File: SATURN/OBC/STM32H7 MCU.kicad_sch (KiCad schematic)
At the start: 16 parts, among them IC1 STM32H735AGI6, IC2 STM32H735AGI6

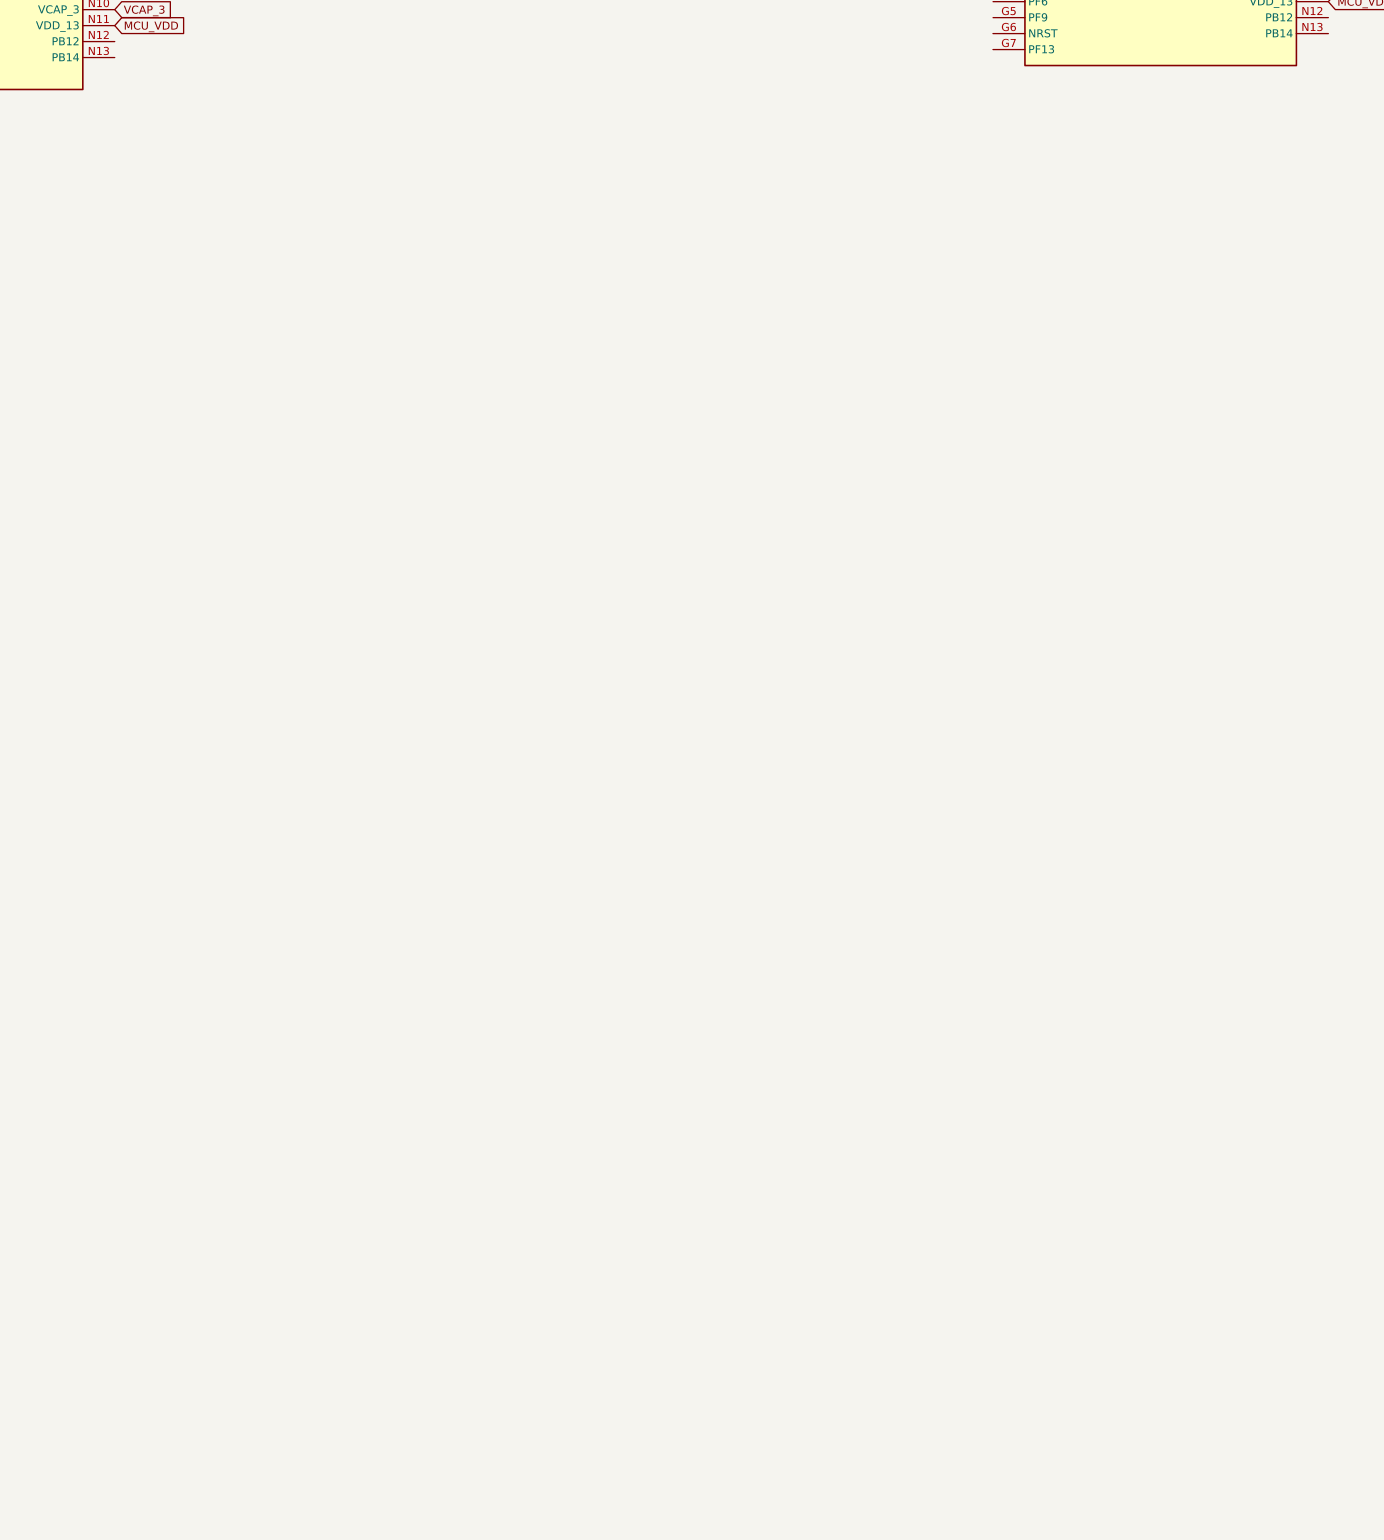
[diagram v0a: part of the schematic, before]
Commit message: a
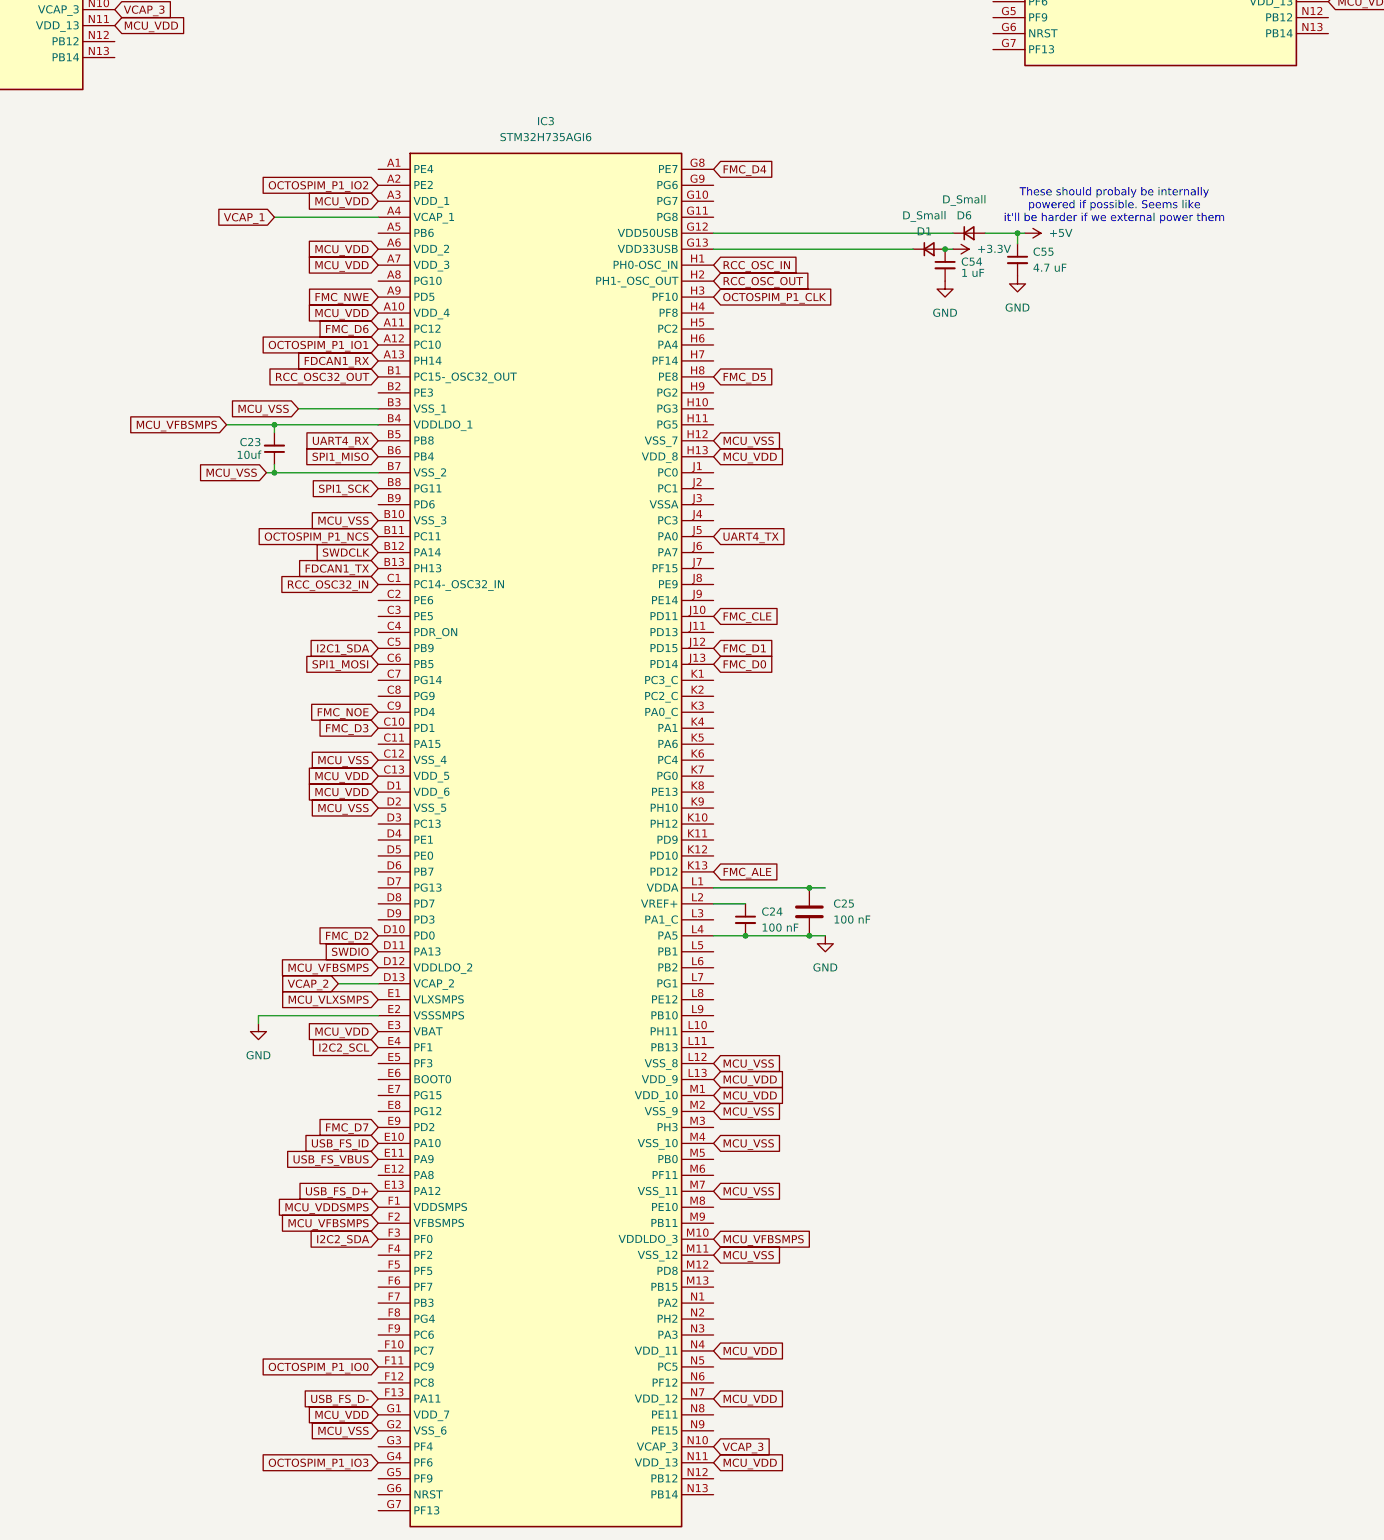
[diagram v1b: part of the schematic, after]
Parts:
- added C23: 10uf, Capacitor_SMD:C_0603_1608Metric, symbol Device:C_Small
- added C24: 100 nF, symbol Device:C_Small
- added C25: 100 nF, symbol Device:C
- added C54: 1 uF, symbol Device:C_Small
- added C55: 4.7 uF, symbol Device:C_Small
- added D1, D6: D_Small, symbol Device:D_Small
- added IC3: STM32H735AGI6, Gabriel_footprints:BGA169C50P13X13_700X700X60, symbol STM32H735AGI6:STM32H735AGI6
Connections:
- net +3.3V: now also C54.1, D1.2 (A)
- net +5V: now also C55.1, D6.2 (A)
- net GND: now also C24.2, C25.2, C54.2, C55.2, IC3.E2 (VSSSMPS), IC3.L4 (PA5)
- net MCU_VDD: now also IC3.A10 (VDD_4), IC3.A3 (VDD_1), IC3.A6 (VDD_2), IC3.A7 (VDD_3), IC3.C13 (VDD_5), IC3.D1 (VDD_6), IC3.E3 (VBAT), IC3.G1 (VDD_7), IC3.H13 (VDD_8), IC3.L13 (VDD_9), IC3.M1 (VDD_10), IC3.N11 (VDD_13), IC3.N4 (VDD_11), IC3.N7 (VDD_12)
- net MCU_VDDSMPS: now also IC3.F1 (VDDSMPS)
- net MCU_VFBSMPS: now also C23.2, IC3.B4 (VDDLDO_1), IC3.D12 (VDDLDO_2), IC3.F2 (VFBSMPS), IC3.M10 (VDDLDO_3)
- net MCU_VLXSMPS: now also IC3.E1 (VLXSMPS)
- net MCU_VSS: now also C23.1, IC3.B10 (VSS_3), IC3.B3 (VSS_1), IC3.B7 (VSS_2), IC3.C12 (VSS_4), IC3.D2 (VSS_5), IC3.G2 (VSS_6), IC3.H12 (VSS_7), IC3.L12 (VSS_8), IC3.M11 (VSS_12), IC3.M2 (VSS_9), IC3.M4 (VSS_10), IC3.M7 (VSS_11)
- net SWDCLK: now also IC3.B12 (PA14)
- net SWDIO: now also IC3.D11 (PA13)
- net VCAP_1: now also IC3.A4 (VCAP_1)
- net VCAP_2: now also IC3.D13 (VCAP_2)
- net VCAP_3: now also IC3.N10 (VCAP_3)
- new net: C25.1, IC3.L1 (VDDA)
- new net: D1.1 (K), IC3.G13 (VDD33USB)
- new net: D6.1 (K), IC3.G12 (VDD50USB)
- new net: C24.1, IC3.L2 (VREF+)
- new net FDCAN1_RX: IC3.A13 (PH14)
- new net FDCAN1_TX: IC3.B13 (PH13)
- new net FMC_ALE: IC3.K13 (PD12)
- new net FMC_CLE: IC3.J10 (PD11)
- new net FMC_D0: IC3.J13 (PD14)
- new net FMC_D1: IC3.J12 (PD15)
- new net FMC_D2: IC3.D10 (PD0)
- new net FMC_D3: IC3.C10 (PD1)
- new net FMC_D4: IC3.G8 (PE7)
- new net FMC_D5: IC3.H8 (PE8)
- new net FMC_D6: IC3.A11 (PC12)
- new net FMC_D7: IC3.E9 (PD2)
- new net FMC_NOE: IC3.C9 (PD4)
- new net FMC_NWE: IC3.A9 (PD5)
- new net I2C1_SDA: IC3.C5 (PB9)
- new net I2C2_SCL: IC3.E4 (PF1)
- new net I2C2_SDA: IC3.F3 (PF0)
- new net OCTOSPIM_P1_CLK: IC3.H3 (PF10)
- new net OCTOSPIM_P1_IO0: IC3.F11 (PC9)
- new net OCTOSPIM_P1_IO1: IC3.A12 (PC10)
- new net OCTOSPIM_P1_IO2: IC3.A2 (PE2)
- new net OCTOSPIM_P1_IO3: IC3.G4 (PF6)
- new net OCTOSPIM_P1_NCS: IC3.B11 (PC11)
- new net RCC_OSC32_IN: IC3.C1 (PC14-_OSC32_IN)
- new net RCC_OSC32_OUT: IC3.B1 (PC15-_OSC32_OUT)
- new net RCC_OSC_IN: IC3.H1 (PH0-OSC_IN)
- new net RCC_OSC_OUT: IC3.H2 (PH1-_OSC_OUT)
- new net SPI1_MISO: IC3.B6 (PB4)
- new net SPI1_MOSI: IC3.C6 (PB5)
- new net SPI1_SCK: IC3.B8 (PG11)
- new net UART4_RX: IC3.B5 (PB8)
- new net UART4_TX: IC3.J5 (PA0)
- new net USB_FS_D+: IC3.E13 (PA12)
- new net USB_FS_D-: IC3.F13 (PA11)
- new net USB_FS_ID: IC3.E10 (PA10)
- new net USB_FS_VBUS: IC3.E11 (PA9)
